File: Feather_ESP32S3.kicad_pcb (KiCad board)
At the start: 2 copper layers, 50.8 x 22.9 mm, 19 parts, among them J1 Conn_01x02, J1 feather long, J2 feather short, Q1 AO3401A, SW1 SW_Push, U1 ESP32-S3-MINI-1, U2 LGS4056H, U3 RT9013-xxGB

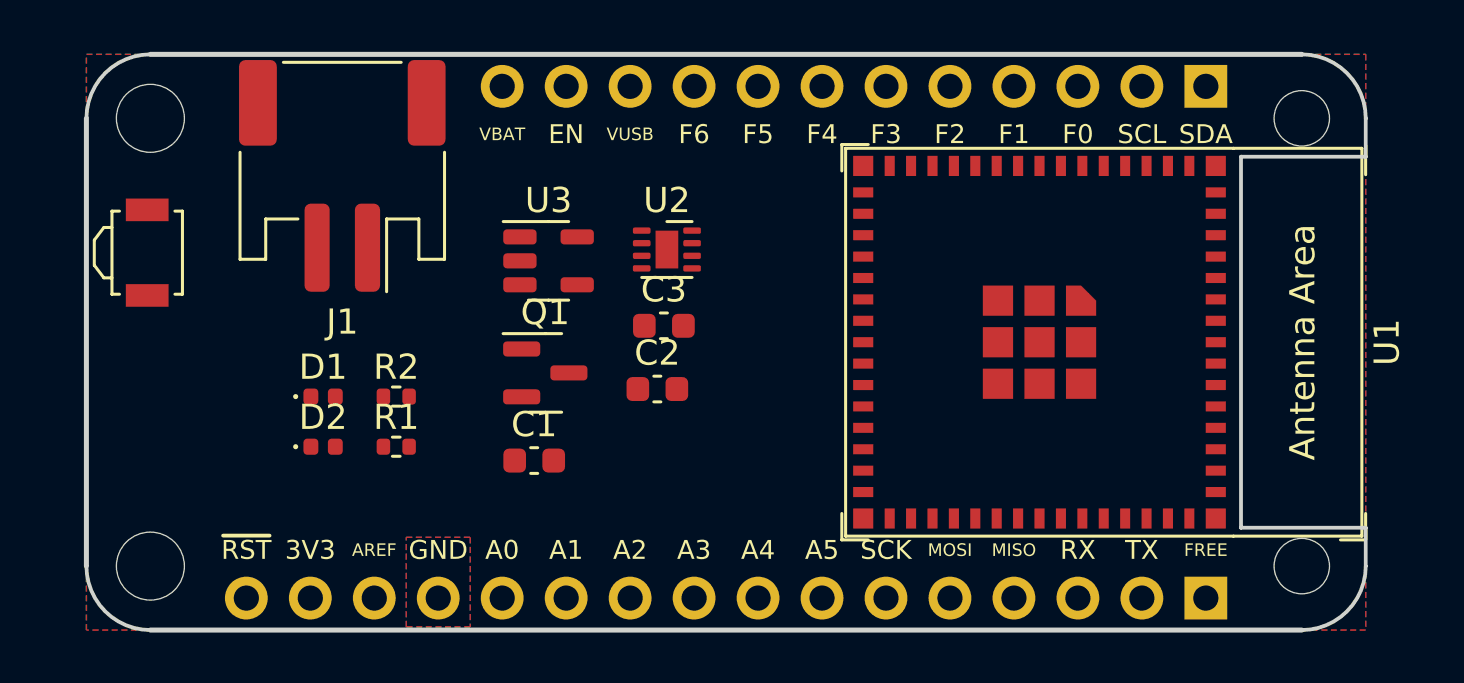
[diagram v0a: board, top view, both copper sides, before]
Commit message: Latest HW
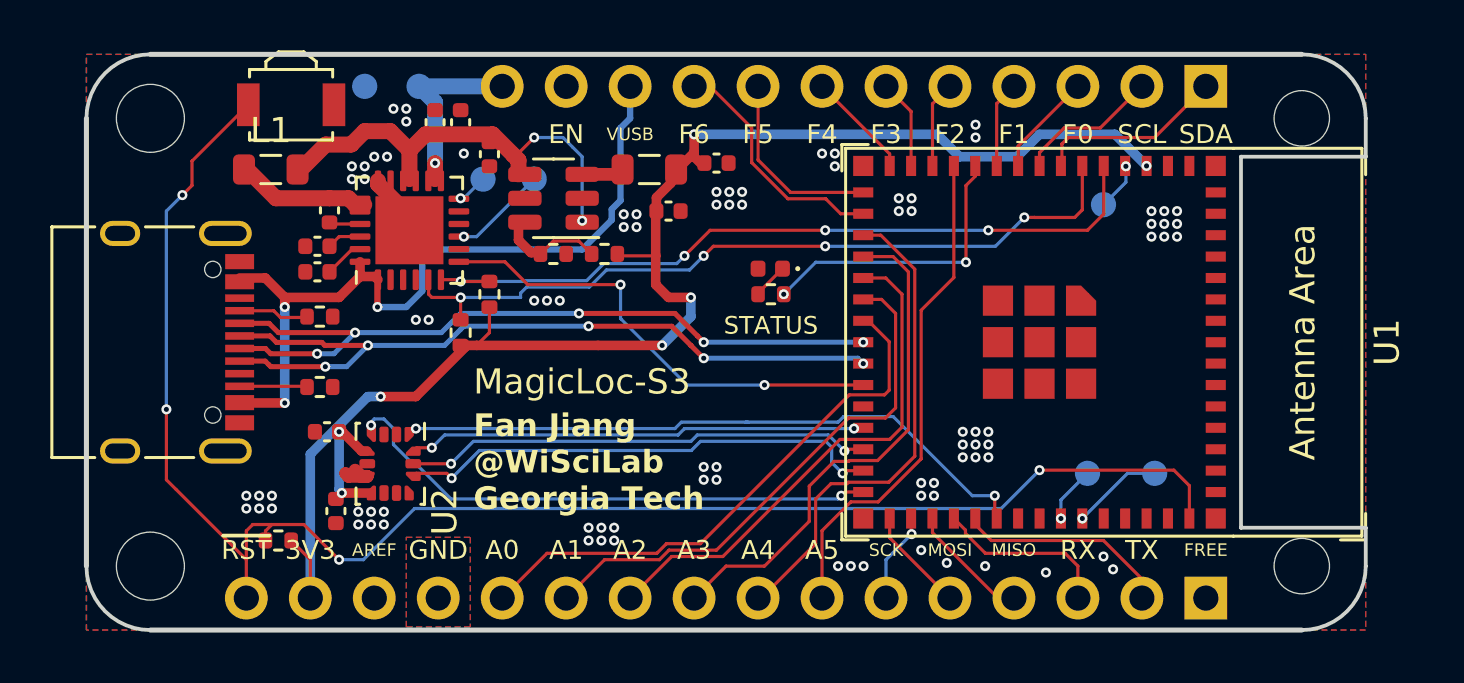
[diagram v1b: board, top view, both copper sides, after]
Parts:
- removed D2: LED, LED_SMD:LED_0402_1005Metric
- removed Q1: AO3401A, Package_TO_SOT_SMD:SOT-23
- added C10: 4.7uF 10V, Capacitor_SMD:C_0402_1005Metric, F.Cu at (41.4, 29.4)
- added C4: 47nF, Capacitor_SMD:C_0402_1005Metric, F.Cu at (35.1, 31.6)
- added C5: 4.7uF, Capacitor_SMD:C_0402_1005Metric, F.Cu at (34.6, 33.0)
- added C6: 10uF, Capacitor_SMD:C_0402_1005Metric, F.Cu at (39.2, 28.1)
- added C7: 10uF, Capacitor_SMD:C_0402_1005Metric, F.Cu at (40.3, 28.1)
- added C8: 100nF, Capacitor_SMD:C_0402_1005Metric, F.Cu at (35.0, 40.4)
- added C9: 100nF, Capacitor_SMD:C_0402_1005Metric, F.Cu at (35.3, 43.5)
- added L1: 1uH 800mA, Inductor_SMD:L_0805_2012Metric, F.Cu at (32.7, 30.0)
- added L2: 2.2uH 800mA 25mOhm, Inductor_SMD:L_0805_2012Metric, F.Cu at (47.8, 30.0)
- added R3: 10k, Resistor_SMD:R_0402_1005Metric, F.Cu at (41.4, 34.9)
- added R4: 10k, Resistor_SMD:R_0402_1005Metric, F.Cu at (40.3, 36.5)
- added R5: 450k 1%, Resistor_SMD:R_0402_1005Metric, F.Cu at (46.0, 33.3)
- added R6: 100k 1%, Resistor_SMD:R_0402_1005Metric, F.Cu at (43.9, 33.3)
- added R7: 10k, Resistor_SMD:R_0402_1005Metric, F.Cu at (33.0, 44.7)
- added R8: 750, Resistor_SMD:R_0402_1005Metric, F.Cu at (52.6, 34.9)
- added TP1: TestPoint, TestPoint:TestPoint_Pad_D1.0mm, B.Cu at (43.2, 30.4)
- added TP2: TestPoint, TestPoint:TestPoint_Pad_D1.0mm, B.Cu at (41.1, 30.4)
- added TP3: BAT+, TestPoint:TestPoint_Pad_D1.0mm, B.Cu at (38.6, 26.7)
- added TP4: TestPoint, TestPoint:TestPoint_Pad_D1.0mm, B.Cu at (36.4, 26.7)
- added TP5: TestPoint, TestPoint:TestPoint_Pad_D1.0mm, B.Cu at (65.8, 31.4)
- added TP6: TestPoint, TestPoint:TestPoint_Pad_D1.0mm, B.Cu at (65.2, 42.0)
- added TP7: TestPoint, TestPoint:TestPoint_Pad_D1.0mm, B.Cu at (67.8, 42.0)
- added U4: SGM41511, Package_DFN_QFN:QFN-24-1EP_4x4mm_P0.5mm_EP2.7x2.7mm, F.Cu at (38.2, 32.4)
- C1: footprint Capacitor_SMD:C_0603_1608Metric -> Capacitor_SMD:C_0402_1005Metric
- C2: value 0.1uF -> 10uF 10V; footprint Capacitor_SMD:C_0603_1608Metric -> Capacitor_SMD:C_0402_1005Metric
- C3: value 10uF -> 100nF; footprint Capacitor_SMD:C_0603_1608Metric -> Capacitor_SMD:C_0402_1005Metric
- J1: value Conn_01x02 -> U262-16XN-4BVC11; footprint Connector_JST:JST_PH_S2B-PH-SM4-TB_1x02-1MP_P2.00mm_Horizontal -> Connector_USB:USB_C_Receptacle_XKB_U262-16XN-4BVC11
- R1, R2: value 2k -> 5.1k
- U2: value LGS4056H -> LSM6DSOTR; footprint Package_DFN_QFN:DFN-8-1EP_2x2mm_P0.5mm_EP0.9x1.5mm -> Package_LGA:LGA-14_3x2.5mm_P0.5mm_LayoutBorder3x4y_JLC
- U3: value RT9013-xxGB -> TLV62569DDC; footprint Package_TO_SOT_SMD:SOT-23-5 -> Package_TO_SOT_SMD:SOT-23-6
- moved D1 18.5 mm to (52.6, 33.9), turned to 180 degrees
- moved U2 13.9 mm to (37.5, 41.7), turned to -90 degrees
- moved C1 11.4 mm to (34.6, 34.0)
- moved J1 10.2 mm to (27.8, 36.8), turned to -90 degrees
- moved C2 9.27 mm to (50.4, 29.7)
- moved SW1 8.19 mm to (33.5, 27.4), turned to 0 degrees
- moved R1 5.99 mm to (34.7, 35.8)
- moved C3 4.56 mm to (48.5, 31.6)
- moved R2 3.06 mm to (34.7, 38.6)
- moved U3 2.49 mm to (43.9, 31.1), turned to 180 degrees
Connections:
- net /BAT_PROG renamed /ESP_IMU/SDX
- C1 pad 2: VBUS -> Net-(U4-PMID)
- C2 pad 1: GND -> +3V3
- C2 pad 2: VBUS -> GND
- C3 pad 1: GND -> +3V3
- C3 pad 2: /VBAT -> GND
- D1 pad 1: Net-(D1-Pad1) -> Net-(D1-K)
- D1 pad 2: Net-(D1-Pad2) -> GND
- J2 pad 10: /VUSB -> VBUS
- R1 pad 1: VBUS -> Net-(J1-CC1)
- R1 pad 2: Net-(D1-Pad2) -> GND
- R2 pad 1: VBUS -> Net-(J1-CC2)
- R2 pad 2: Net-(D2-Pad2) -> GND
- U1 pad 11: unconnected-(U1-Pad11) -> /STATUS_LED
- U1 pad 25: unconnected-(U1-Pad25) -> /~{INT}_BMS
- U1 pad 27: unconnected-(U1-Pad27) -> /IMU_MOSI
- U1 pad 28: unconnected-(U1-Pad28) -> /IMU_SCLK
- U1 pad 29: unconnected-(U1-Pad29) -> /IMU_CS
- U1 pad 30: unconnected-(U1-Pad30) -> /IMU_INT1
- U1 pad 36: unconnected-(U1-Pad36) -> /IMU_MISO
- U1 pad 39: unconnected-(U1-Pad39) -> /ESP_U0_TXD
- U1 pad 40: unconnected-(U1-Pad40) -> /ESP_U0_RXD
- U1 pad 5: unconnected-(U1-Pad5) -> /SDA_BMS
- U1 pad 6: unconnected-(U1-Pad6) -> /SCL_BMS
- U2 pad 1: /BAT_TEMP -> /IMU_MISO
- U2 pad 3: GND -> /ESP_IMU/SCX
- U2 pad 4: VBUS -> /IMU_INT1
- U2 pad 5: /VBAT -> +3V3
- U2 pad 6: Net-(D2-Pad1) -> GND
- U2 pad 7: Net-(D1-Pad1) -> GND
- U2 pad 8: VBUS -> +3V3
- U2 pad 9: (no net) -> /ESP_IMU/INT2
- U3 pad 1: VBUS -> VCC
- U3 pad 3: VBUS -> Net-(U3-SW)
- U3 pad 4: GND -> VCC
- U3 pad 5: +3V3 -> unconnected-(U3-PG-Pad5)
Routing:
- net /~{RST}: track 0.00 -> 65.3 mm, vias 0 -> 4
- net +3V3: track 0.00 -> 63.2 mm, vias 0 -> 7
- net /ESP_USB_DP: track 0.00 -> 31.4 mm, vias 0 -> 5
- net /SCL_BMS: track 0.00 -> 30.8 mm, vias 0 -> 4
- net /ESP_USB_DN: track 0.00 -> 30.7 mm, vias 0 -> 5
- net /SDA_BMS: track 0.00 -> 30.5 mm, vias 0 -> 4
- net VBUS: track 0.00 -> 30.4 mm, vias 0 -> 3
- net /IMU_MISO: track 0.00 -> 25.9 mm, vias 0 -> 2
- net /A0: track 0.00 -> 22.1 mm
- net /IMU_INT1: track 0.00 -> 21.9 mm, vias 0 -> 2
- net /A1: track 0.00 -> 21.5 mm
- net /A2: track 0.00 -> 20.7 mm
- net /A3: track 0.00 -> 20.4 mm
- net /A5: track 0.00 -> 20.0 mm
- net /A4: track 0.00 -> 19.6 mm
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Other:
- rule pad_to_mask_clearance: 0.051 -> 0
- board text added: "Fan Jiang @WiSciLab Georgia Tech"
- board text added: "MagicLoc-S3"
- board text added: "STATUS"
- board text removed: "VBAT"
